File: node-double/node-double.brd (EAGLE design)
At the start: 35.1 x 24.3 mm, 31 parts, among them IC1 TP4056, U1 ATMEGA328P_TQFP, U2 3.3V/150mA

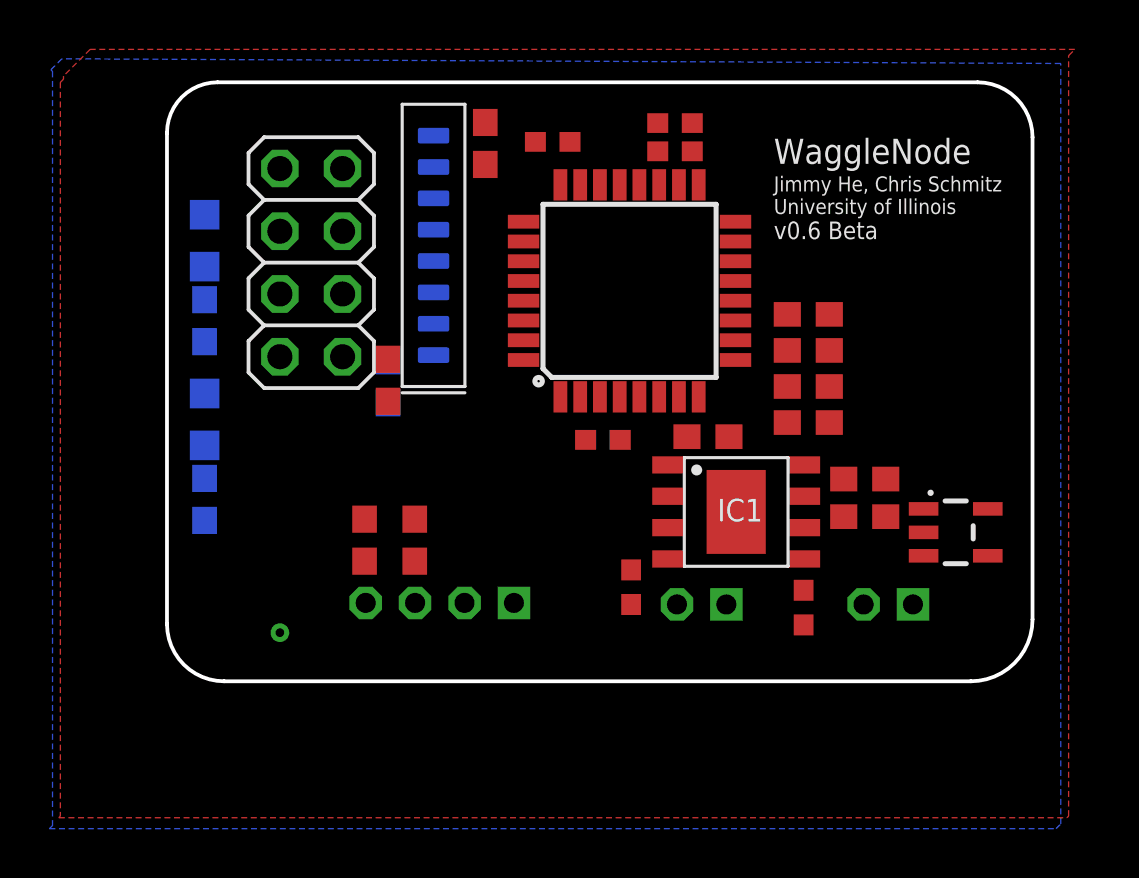
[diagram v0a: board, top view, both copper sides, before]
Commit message: Routing & VCC Optimization
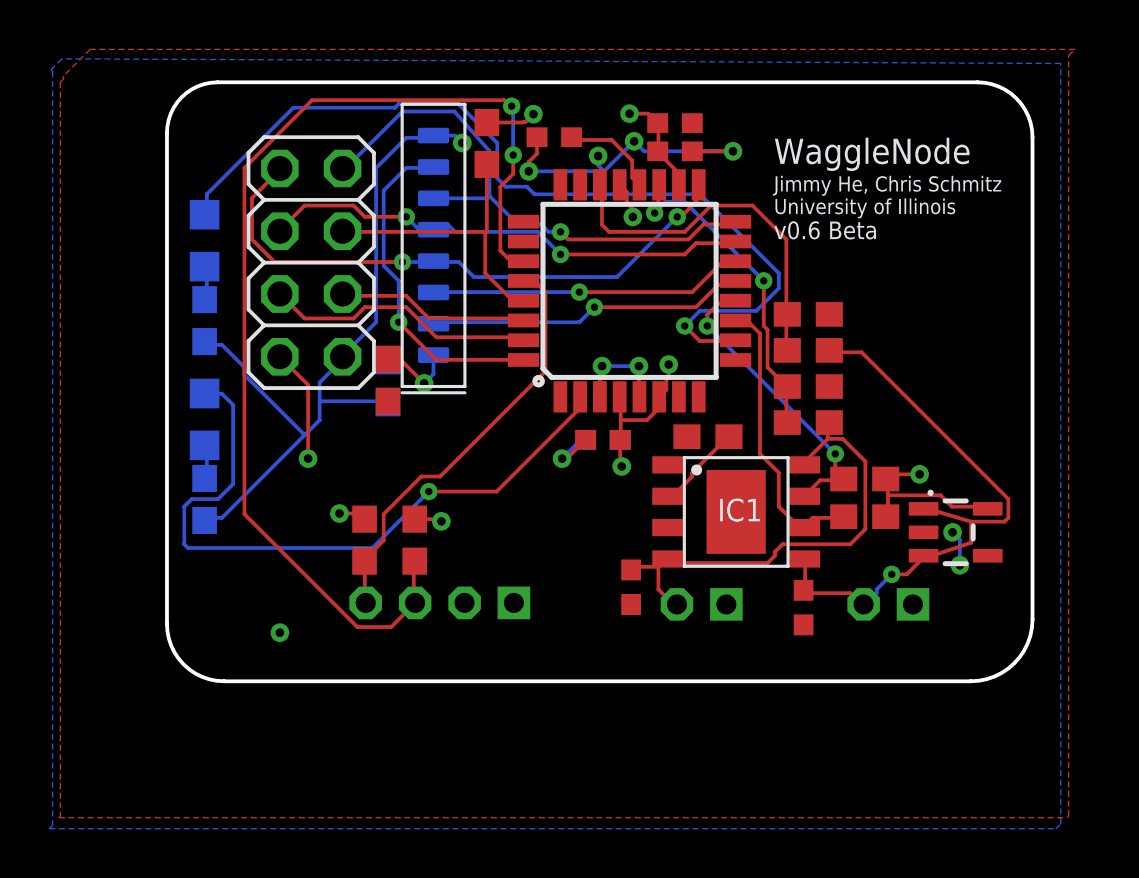
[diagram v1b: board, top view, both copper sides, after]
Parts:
- moved C1 0.20 mm to (36.3, 42.5)
- moved R1 0.06 mm to (33.6, 42.3)
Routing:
- net GND: track 0.00 -> 52.7 mm, vias 0 -> 11
- net SDA/A4: track 0.00 -> 44.3 mm, vias 0 -> 2
- net D6: track 0.00 -> 36.6 mm, vias 0 -> 1
- net VCC: track 0.00 -> 30.1 mm, vias 0 -> 9
- net D4: track 0.00 -> 27.3 mm, vias 0 -> 1
- net VBAT: track 0.00 -> 24.3 mm, vias 0 -> 1
- net SCK/13: track 0.00 -> 24.0 mm, vias 0 -> 2
- net MISO/12: track 0.00 -> 22.7 mm, vias 0 -> 1
- net MOSI/11: track 0.00 -> 20.1 mm, vias 0 -> 2
- net VIN: track 0.00 -> 19.9 mm
- net SCL/A5: track 0.00 -> 17.2 mm
- net A7: track 0.00 -> 14.8 mm
- net D2: track 0.00 -> 13.7 mm, vias 0 -> 1
- net A6: track 0.00 -> 13.3 mm, vias 0 -> 2
- net D9: track 0.00 -> 13.0 mm, vias 0 -> 1
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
